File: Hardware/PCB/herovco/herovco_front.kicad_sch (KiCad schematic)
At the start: 72 parts, among them U1 TL074, U2 TL072, U3 AS3340A, U4 LM4040BIZ-5, U5 LM4040BIZ-5, U6 L79L05_TO92

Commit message: Initial BOM; DNF the test points; README typo
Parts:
- TP1, TP3, TP5: Config (none) -> DNF
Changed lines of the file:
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@@
+      (effects (font (size 1.27 1.27)) hide)
+    )
+    (property "Config" "DNF" (id 4) (at 158.75 91.44 0)
       (effects (font (size 1.27 1.27)) hide)
     )
@@
       (effects (font (size 1.27 1.27)) hide)
     )
+    (property "Config" "DNF" (id 4) (at 181.61 91.44 0)
+      (effects (font (size 1.27 1.27)) hide)
+    )
     (pin "1")
   )
@@
       (effects (font (size 1.27 1.27)) hide)
     )
+    (property "Config" "DNF" (id 4) (at 204.47 91.44 0)
+      (effects (font (size 1.27 1.27)) hide)
+    )

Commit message: Correct slide switch footprint; use TO-92 wide for regulator
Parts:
- U6: footprint Package_TO_SOT_THT:TO-92_Inline -> ao_tht:TO-92_Inline_Wide
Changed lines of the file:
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@@
     (property "Reference" "U6" (id 0) (at 241.3 47.1932 0))
     (property "Value" "L79L05_TO92" (id 1) (at 241.3 49.5046 0))
-    (property "Footprint" "Package_TO_SOT_THT:TO-92_Inline" (id 2) (at 241.3 48.26 0)
+    (property "Footprint" "ao_tht:TO-92_Inline_Wide" (id 2) (at 241.3 48.26 0)
       (effects (font (size 1.27 1.27) italic) hide)
     )

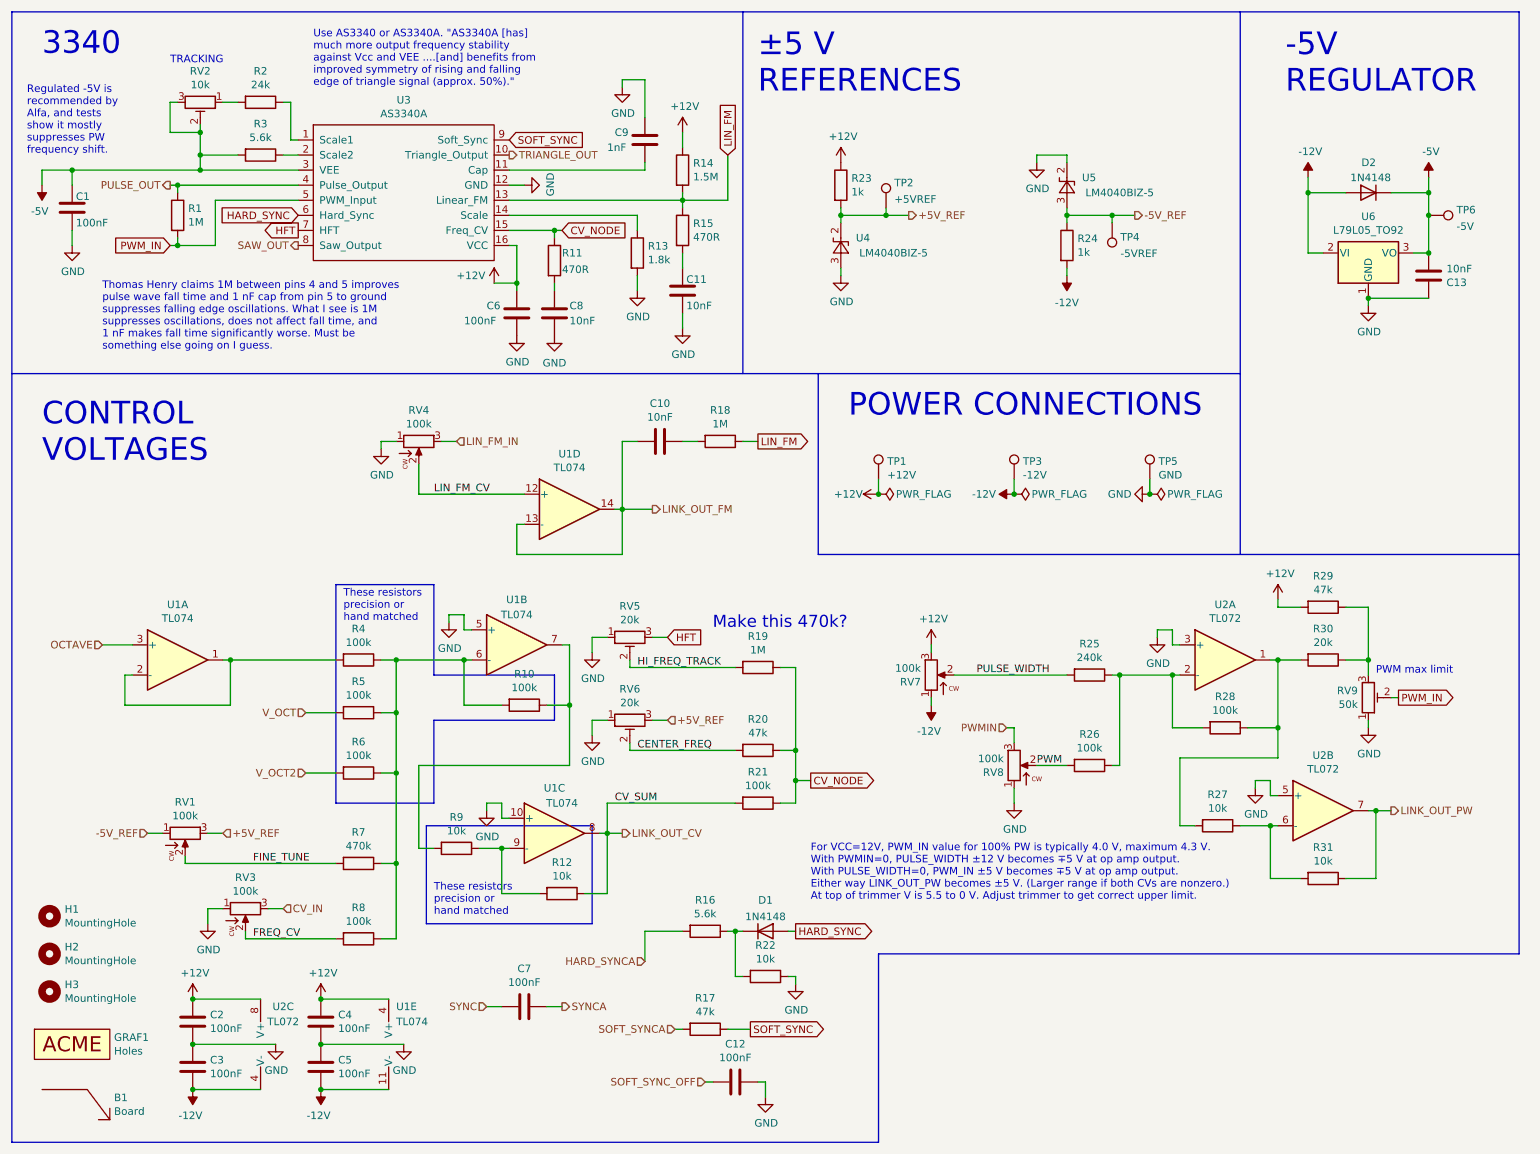
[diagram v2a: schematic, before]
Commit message: Use uninverted PW CV
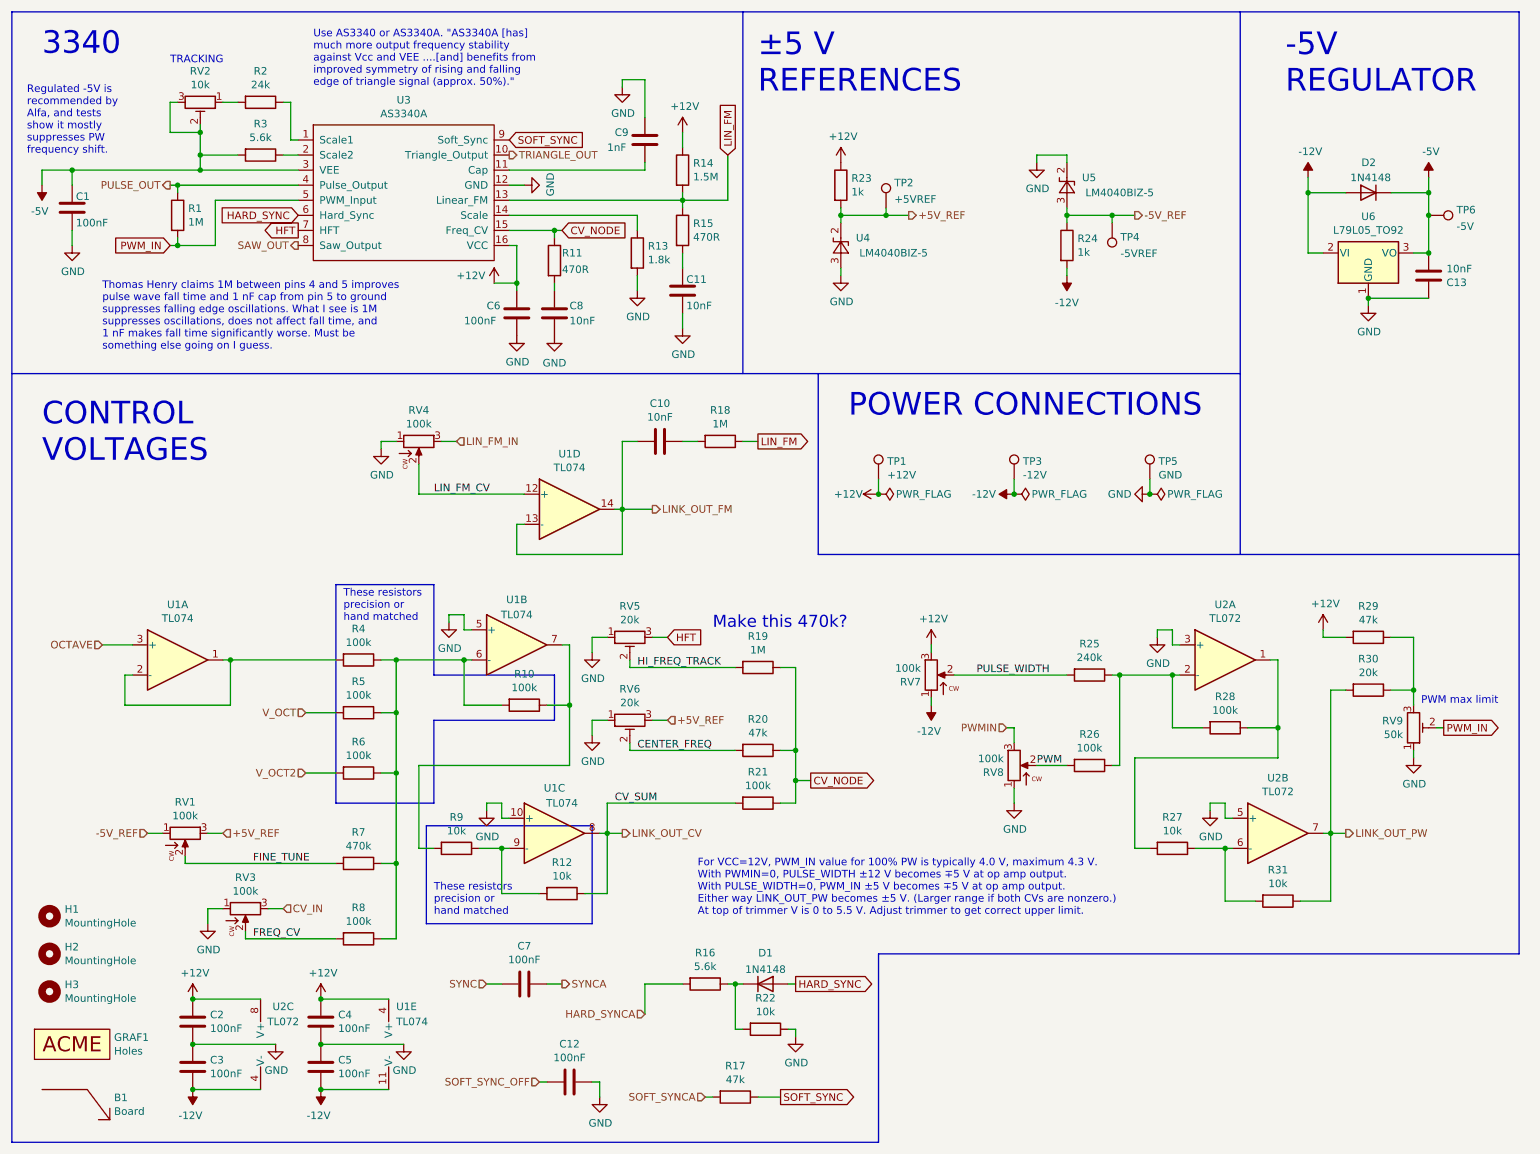
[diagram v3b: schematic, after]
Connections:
- net LINK_OUT_PW: now also R30.2
- net at R27.2, R28.1, U2.1: no longer R30.2
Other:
- note added: "For VCC=12V, PWM_IN value for 100% PW is typically 4.0 V, maximum 4.3 V. With PWMIN=0, PULSE_WIDTH ±12 V becomes ∓5 V at op amp output. With PULSE_WIDTH=0, PWM_IN ±5 V becomes ∓5 V at op amp output. Either way LINK_OUT_PW becomes ±5 V. (Larger range if both CVs are nonzero.) At top of trimmer V is 0 to 5.5 V. Adjust trimmer to get correct upper limit."
- note removed: "For VCC=12V, PWM_IN value for 100% PW is typically 4.0 V, maximum 4.3 V. With PWMIN=0, PULSE_WIDTH ±12 V becomes ∓5 V at op amp output. With PULSE_WIDTH=0, PWM_IN ±5 V becomes ∓5 V at op amp output. Either way LINK_OUT_PW becomes ±5 V. (Larger range if both CVs are nonzero.) At top of trimmer V is 5.5 to 0 V. Adjust trimmer to get correct upper limit."
- moved on the sheet: C12, C7, D1, R16, R17, R22, R27, R29, R30, R31, RV9, U2B

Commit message: Revert "Use uninverted PW CV"
This reverts commit afeb33e5ee15cb89f0e577c33928166723912ed3.
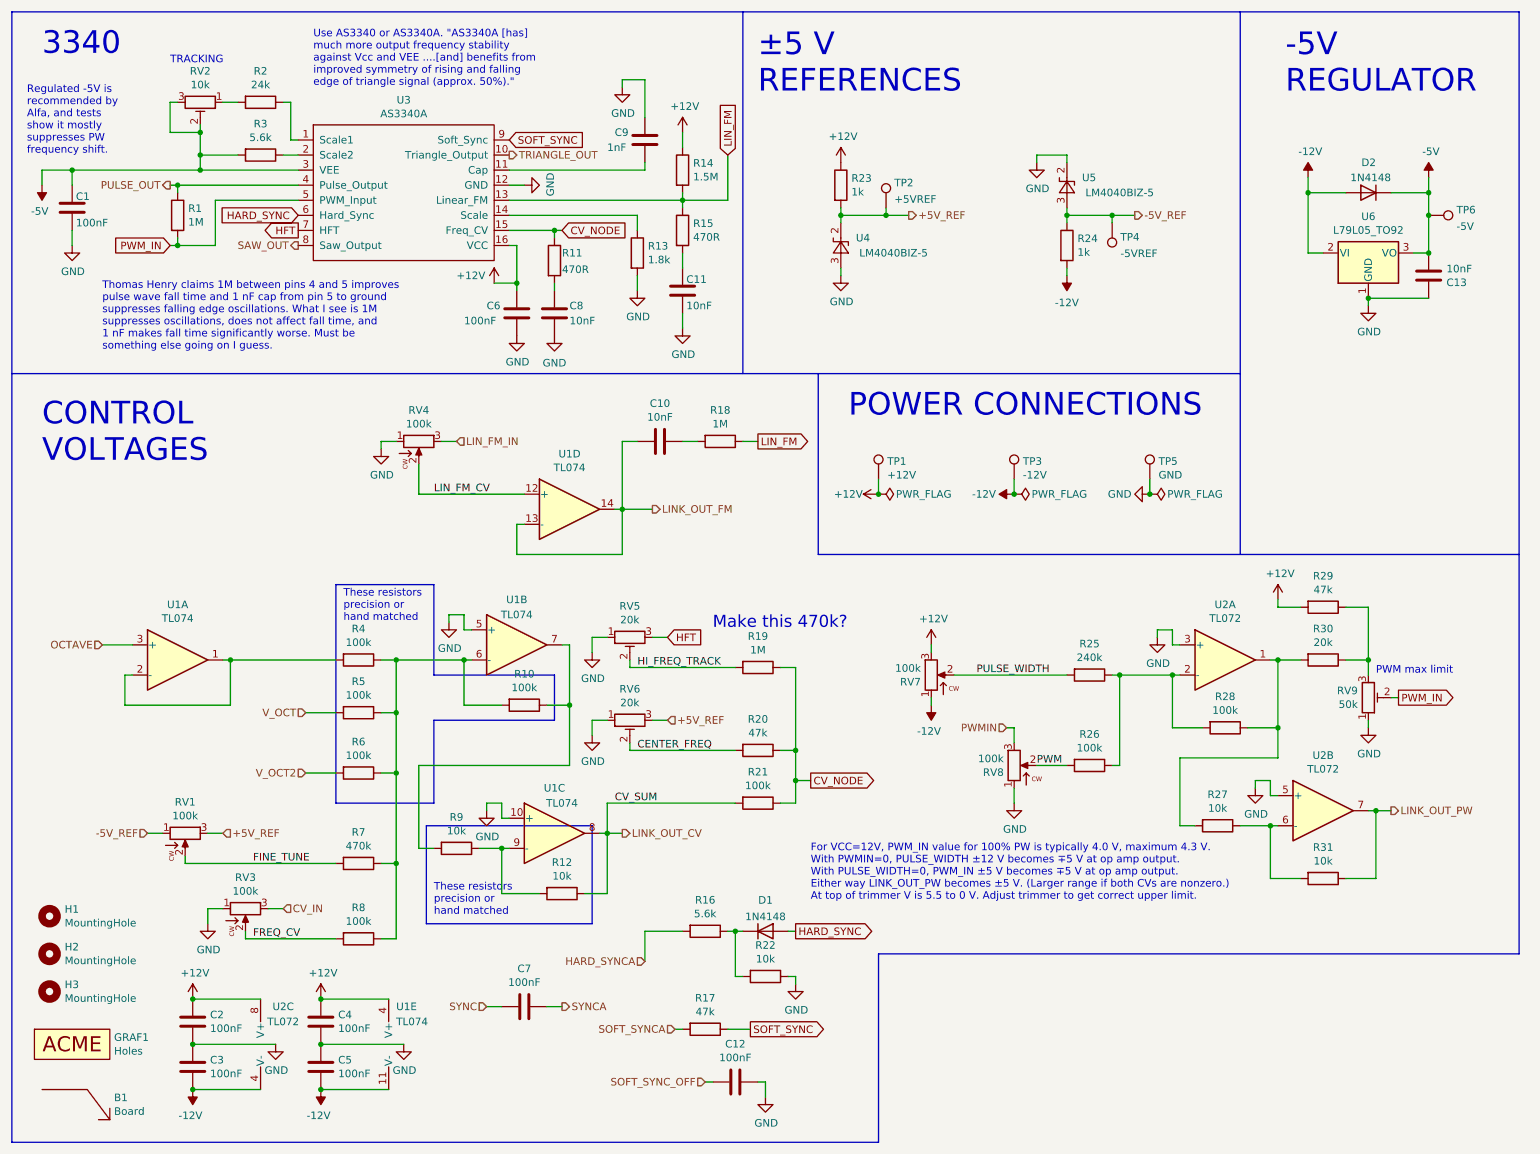
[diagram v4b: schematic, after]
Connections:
- net LINK_OUT_PW: no longer R30.2
- net at R27.2, R28.1, U2.1: now also R30.2
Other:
- note added: "For VCC=12V, PWM_IN value for 100% PW is typically 4.0 V, maximum 4.3 V. With PWMIN=0, PULSE_WIDTH ±12 V becomes ∓5 V at op amp output. With PULSE_WIDTH=0, PWM_IN ±5 V becomes ∓5 V at op amp output. Either way LINK_OUT_PW becomes ±5 V. (Larger range if both CVs are nonzero.) At top of trimmer V is 5.5 to 0 V. Adjust trimmer to get correct upper limit."
- note removed: "For VCC=12V, PWM_IN value for 100% PW is typically 4.0 V, maximum 4.3 V. With PWMIN=0, PULSE_WIDTH ±12 V becomes ∓5 V at op amp output. With PULSE_WIDTH=0, PWM_IN ±5 V becomes ∓5 V at op amp output. Either way LINK_OUT_PW becomes ±5 V. (Larger range if both CVs are nonzero.) At top of trimmer V is 0 to 5.5 V. Adjust trimmer to get correct upper limit."
- moved on the sheet: C12, C7, D1, R16, R17, R22, R27, R29, R30, R31, RV9, U2B
